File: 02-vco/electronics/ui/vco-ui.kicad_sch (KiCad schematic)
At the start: 32 parts, among them J1 Conn_01x04, J2 Conn_02x05_Odd_Even, J3 Conn_02x03_Odd_Even, J4 Conn_01x02, J5 Conn_02x02_Counter_Clockwise, J6 Conn_01x06

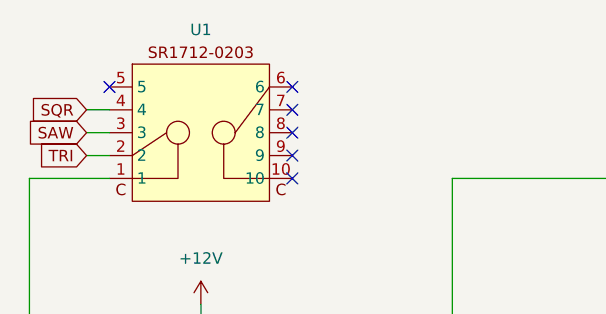
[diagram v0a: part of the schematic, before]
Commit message: Refined VCO core and UI
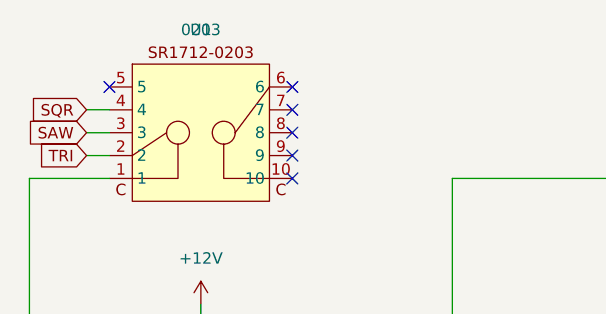
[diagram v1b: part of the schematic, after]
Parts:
- H1, H2, H3, H4, H5: Vendor (none) -> -
- J1: Part URL (none) -> https://mou.sr/4kxE3Vr; Part no. (none) -> 200-SSW10401TMS; Vendor (none) -> Mouser; now in the parts list
- J2: Part URL (none) -> https://mou.sr/4lVCZM9; Part no. (none) -> 200-SSW10501TD; Vendor (none) -> Mouser; now in the parts list
- J3: Part URL (none) -> https://mou.sr/3GIDVEr; Part no. (none) -> 200-SSW10301TD; Vendor (none) -> Mouser; now in the parts list
- J4: Part URL (none) -> https://mou.sr/4lBvdHe; Part no. (none) -> 200-SSW10201TS; Vendor (none) -> Mouser
- J5: Part URL (none) -> https://mou.sr/4eSbYqI; Part no. (none) -> 200-SSW10206TD; Vendor (none) -> Mouser; now in the parts list
- J6: Part URL (none) -> https://mou.sr/4lnf48h; Part no. (none) -> 200-SSW10601TS; Vendor (none) -> Mouser
- JP1: Part URL (none) -> https://mou.sr/451l2py; Part no. (none) -> 200-HTSW10308TSRA; Vendor (none) -> Mouser; now in the parts list
- JP2, JP3: Part URL (none) -> https://mou.sr/4nM6IZz; Part no. (none) -> 200-HTSW10208TSRA; Vendor (none) -> Mouser; now in the parts list
- J_CV1, J_EXTRA_OUT1, J_FM1, J_OUT1, J_PWM1, J_SYNC1: Part URL (none) -> https://www.thonk.co.uk/shop/thonkiconn/; Part no. (none) -> PJ398SM; Vendor (none) -> Thonk
- R1, R4, R5: Vendor (none) -> Mouser
- R2, R3, R6: Part URL (none) -> https://mou.sr/4hEwI4G; Part no. (none) -> 603-MFR-25FRF52100K; Vendor (none) -> Mouser
- R7, R8: Part URL (none) -> https://mou.sr/46cEvF7; Part no. (none) -> 603-MFR-25FRF52-220K; Vendor (none) -> Mouser
- RV_FINE1, RV_PWM1, RV_TUNE1: Part URL (none) -> https://mou.sr/4694GMU; Part no. (none) -> 652-PTV09A4025FB104; Vendor (none) -> Mouser
- U1: value ~ -> 0203; Part No. 105-SR1712F-23NS -> (none); Part URL (none) -> https://mou.sr/3U6bGTk; Part no. (none) -> 105-SR1712F-23NS
